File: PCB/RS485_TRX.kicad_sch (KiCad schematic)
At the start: 8 parts, among them J4 1-770969-0, U5 SN65HVD11HD

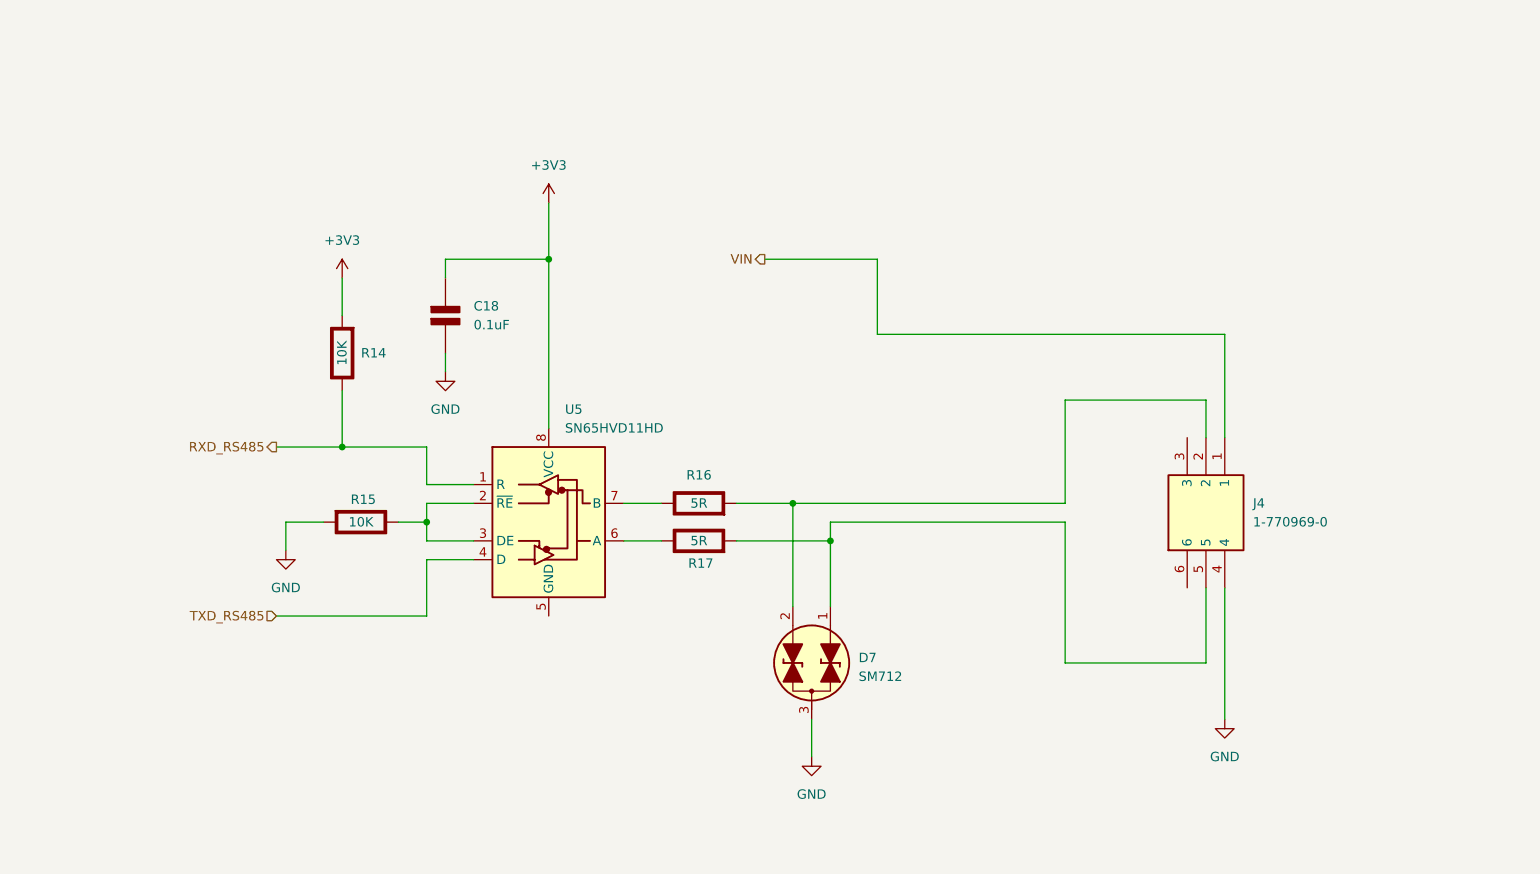
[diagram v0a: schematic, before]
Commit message: Updated PCB
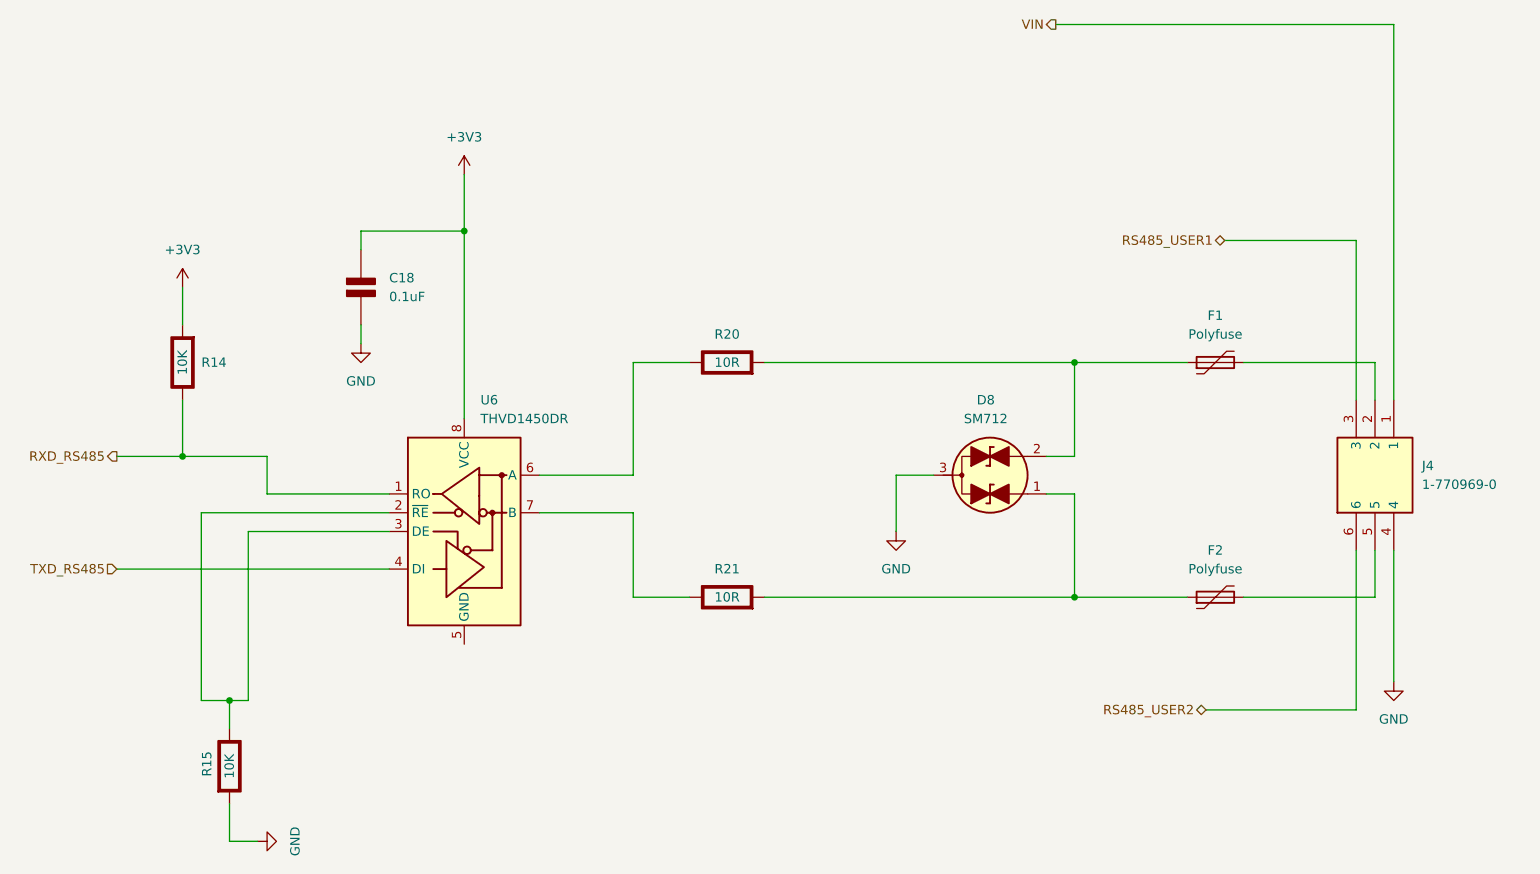
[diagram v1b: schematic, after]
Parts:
- removed D7: SM712, PCM_Package_TO_SOT_SMD_AKL:SOT-23, symbol PCM_Diode_TVS_AKL:SM712
- removed R16, R17: 5R, symbol PCM_Elektuur:R
- removed U5: SN65HVD11HD, Package_SO:SOIC-8_3.9x4.9mm_P1.27mm, symbol Interface_UART:SN65HVD11HD
- added D8: SM712, PCM_Package_TO_SOT_SMD_AKL:SOT-23, symbol PCM_Diode_TVS_AKL:SM712
- added F1, F2: Polyfuse, symbol Device:Polyfuse
- added R20, R21: 10R, symbol PCM_Elektuur:R
- added U6: THVD1450DR, Package_SON:VSON-8-1EP_3x3mm_P0.65mm_EP1.6x2.4mm, symbol Interface_UART:THVD1450DR
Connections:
- net +3V3: now also U6.8 (VCC)
- net GND: now also D8.3 (Com)
- net RXD_RS485: now also U6.1 (RO)
- net TXD_RS485: now also U6.4 (DI)
- net at J4.2: now also F1.2
- net RS485_USER1: now reaches J4.3
- net at J4.5: now also F2.2
- net RS485_USER2: now reaches J4.6
- net at R15.1 (+): now also U6.2 (~{RE}), U6.3 (DE)
- new net: R21.1 (+), U6.7 (B)
- new net: D8.1 (A1), F2.1, R21.2 (-)
- new net: D8.2 (A2), F1.1, R20.2 (-)
- new net: R20.1 (+), U6.6 (A)
